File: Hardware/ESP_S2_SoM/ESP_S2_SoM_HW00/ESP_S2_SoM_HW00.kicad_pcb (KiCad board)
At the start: 6 copper layers, 29.5 x 24.7 mm, 58 parts, among them J101 DF40C-60DP-0.4V(51), J102 Bare PCB USB C, SW401 SW_Push, SW402 SW_Push, U201 BQ24075RGTR, U301 MIC5528-3.3YMT-T5, U401 ESP32-S2FH4, Y601 Crystal_GND24_Small

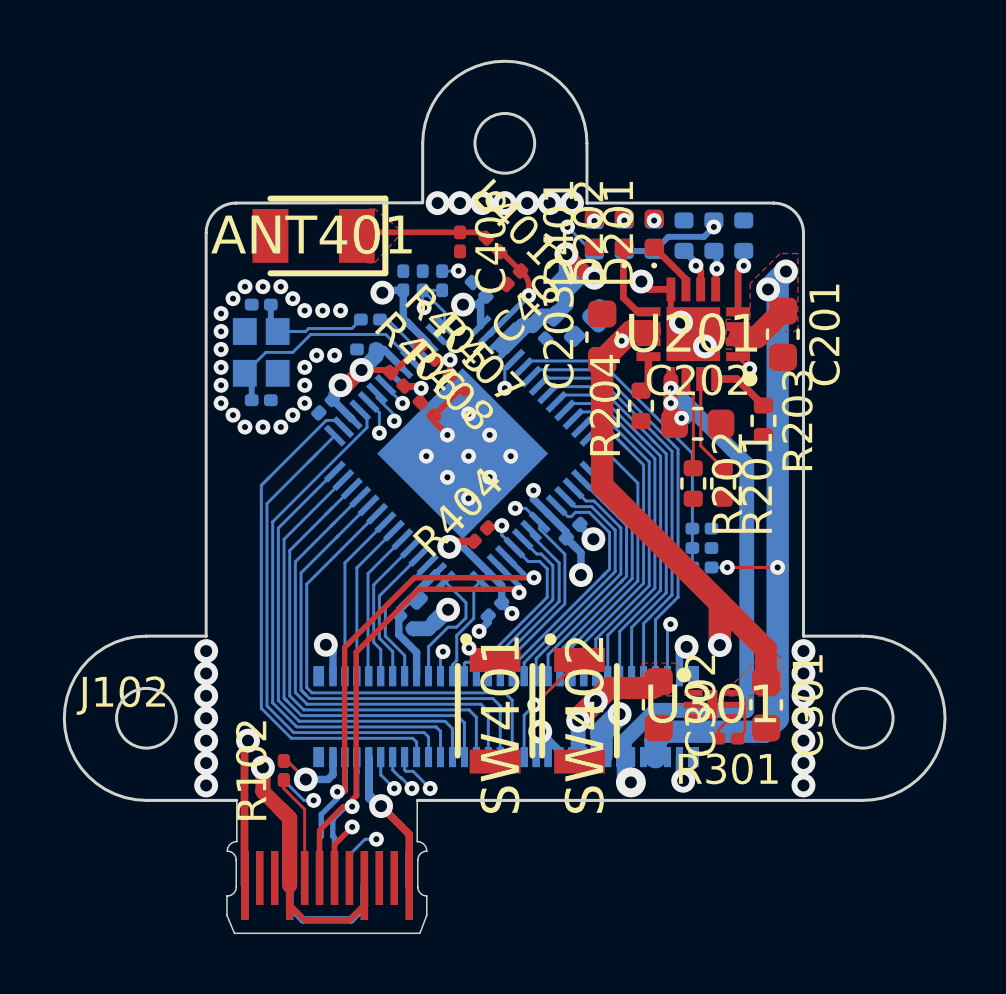
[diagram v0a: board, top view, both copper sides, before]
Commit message: Routing done, ready for prod
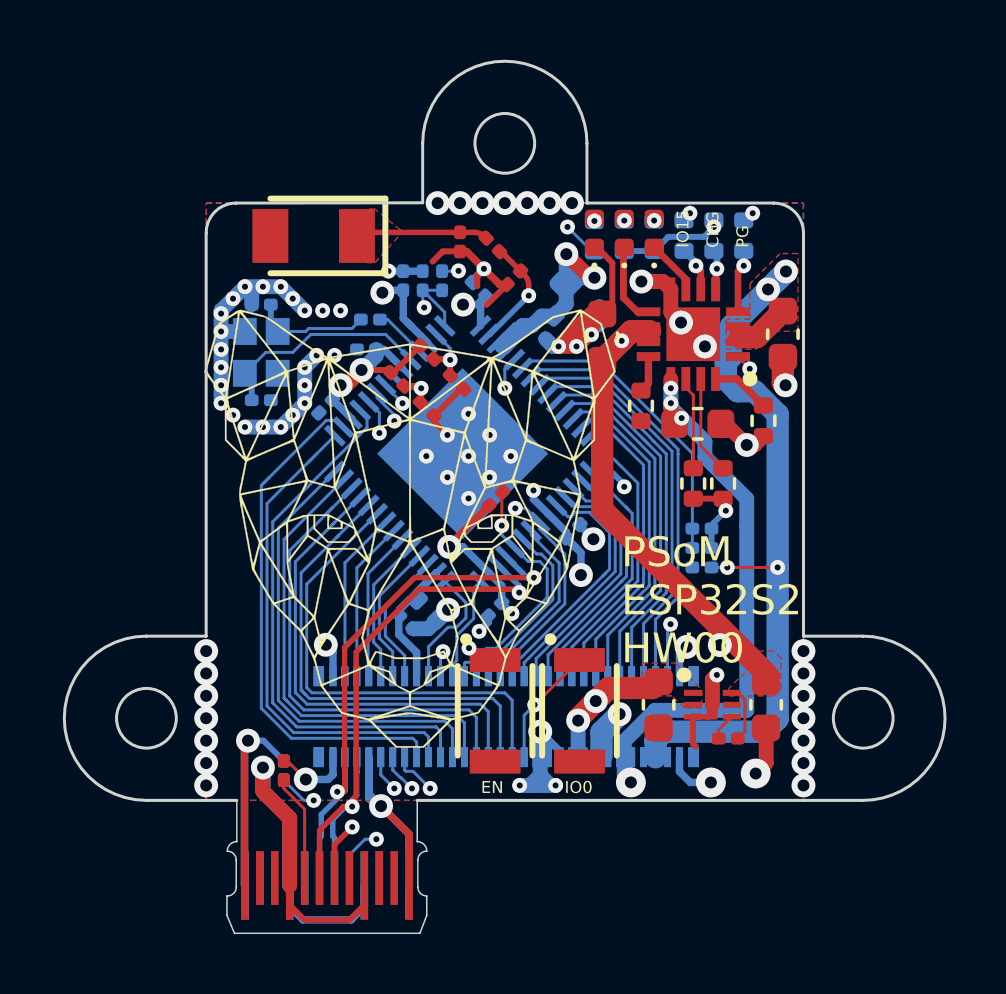
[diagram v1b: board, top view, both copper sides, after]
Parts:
- added G***: LOGO, Component_lib:puma_logo_14mm, F.Cu at (132.8, 99.9)
- moved R404 1.30 mm to (135.7, 98.9)
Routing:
- net GND: track 38.7 -> 90.3 mm, vias 68 -> 83
- net /VSYS: track 35.1 -> 39.0 mm
- net VBUS: track 51.4 -> 49.7 mm
- net /VBAT: track 24.9 -> 26.2 mm
- net +3V3: track 34.5 -> 35.4 mm
- net IO15: track 21.4 -> 20.7 mm
- net IO18: track 7.88 -> 8.51 mm
- added copper zone on B.Cu, net GND
- added copper zone on F.Cu, net GND
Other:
- board text added: "CHG"
- board text added: "EN"
- board text added: "IO0"
- board text added: "IO15"
- board text added: "PG"
- board text added: "PSoM ESP32S2 HW00"
